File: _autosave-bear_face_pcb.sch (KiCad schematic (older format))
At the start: 201 parts, among them J1 GT-USB-7010EN, J2 Conn_02x03_Odd_Even, SW1 RESET, U1 ATmega32U4-AU, U2 SRV05-4, Y1 16MHz

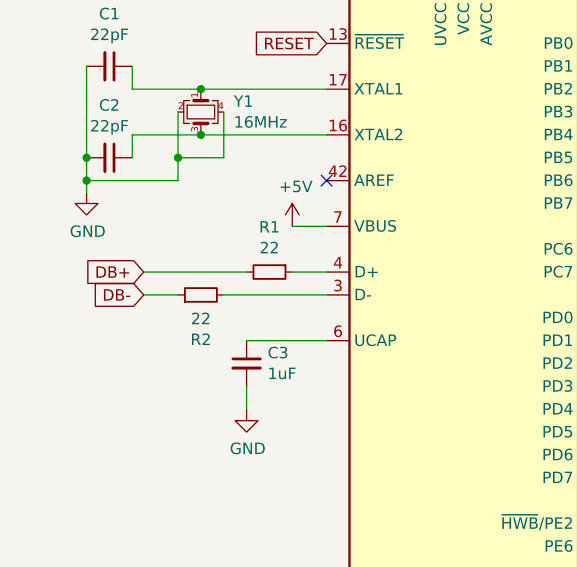
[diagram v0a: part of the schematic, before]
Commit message: initial USB-C commit
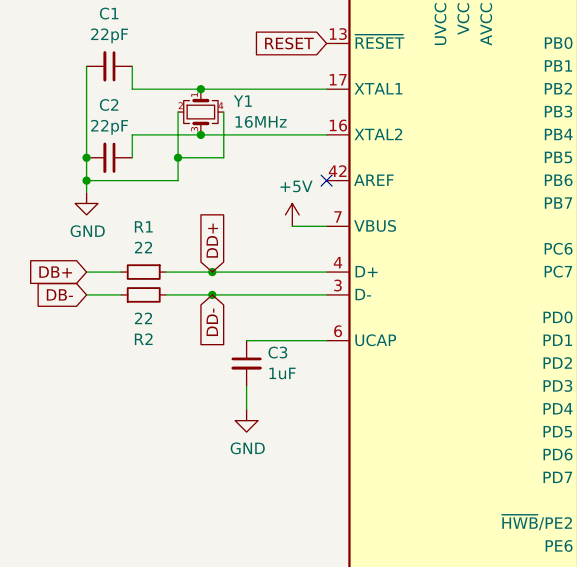
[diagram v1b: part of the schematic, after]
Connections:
- net DD-: now reaches R2.2, U1.3 (D-)
- net DD+: now reaches R1.1, U1.4 (D+)
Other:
- moved on the sheet: R1, R2
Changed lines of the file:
@@
 Text GLabel 5500 5900 2    50   Input ~ 0
 DA+
-Text GLabel 1550 2450 0    50   Input ~ 0
-DB-
 Text GLabel 3300 3500 1    50   Input ~ 0
 LEDPIN
-Text GLabel 950  5150 0    50   Input ~ 0
-DB+
-Text GLabel 950  5250 0    50   Input ~ 0
-DB-
 Wire Wire Line
 	2250 7450 2350 7450
@@
 Wire Wire Line
 	1700 2600 1550 2600
-Text GLabel 1550 2600 0    50   Input ~ 0
-DB+
 Wire Wire Line
 	1700 2250 1700 2600
@@
 L Device:R_Small R1
 U 1 1 66036275
-P 1500 5150
-F 0 "R1" V 1304 5150 50  0000 C CNN
-F 1 "22" V 1395 5150 50  0000 C CNN
-F 2 "Resistor_SMD:R_0805_2012Metric" H 1500 5150 50  0001 C CNN
-F 3 "~" H 1500 5150 50  0001 C CNN
-	1    1500 5150
+P 950 5150
+F 0 "R1" V 754 5150 50  0000 C CNN
+F 1 "22" V 845 5150 50  0000 C CNN
+F 2 "Resistor_SMD:R_0805_2012Metric" H 950 5150 50  0001 C CNN
+F 3 "~" H 950 5150 50  0001 C CNN
+	1    950  5150
 	0    1    1    0
 $EndComp
-Wire Wire Line
-	1750 5150 1600 5150
-Wire Wire Line
-	1400 5150 950  5150
-Wire Wire Line
-	1100 5250 950  5250
-Wire Wire Line
-	1300 5250 1750 5250
 $Comp
 L Device:R_Small R2
 U 1 1 66037A5E
-P 1200 5250
-F 0 "R2" V 1004 5250 50  0000 C CNN
-F 1 "22" V 1095 5250 50  0000 C CNN
-F 2 "Resistor_SMD:R_0805_2012Metric" H 1200 5250 50  0001 C CNN
-F 3 "~" H 1200 5250 50  0001 C CNN
-	1    1200 5250
+P 950 5250
+F 0 "R2" V 754 5250 50  0000 C CNN
+F 1 "22" V 845 5250 50  0000 C CNN
+F 2 "Resistor_SMD:R_0805_2012Metric" H 950 5250 50  0001 C CNN
+F 3 "~" H 950 5250 50  0001 C CNN
+	1    950  5250
 	0    -1   -1   0
 $EndComp
+Text GLabel 700  5250 0    50   Input ~ 0
+DB-
+Text GLabel 700  5150 0    50   Input ~ 0
+DB+
+Text GLabel 1550 2600 0    50   Input ~ 0
+DB+
+Text GLabel 1550 2450 0    50   Input ~ 0
+DB-
+Text GLabel 1250 5150 1    50   Input ~ 0
+DD+
+Wire Wire Line
+	700  5150 850  5150
+Wire Wire Line
+	1050 5150 1250 5150
+Wire Wire Line
+	700  5250 850  5250
+Wire Wire Line
+	1050 5250 1250 5250
+Connection ~ 1250 5150
+Wire Wire Line
+	1250 5150 1750 5150
+Connection ~ 1250 5250
+Wire Wire Line
+	1250 5250 1750 5250
+Text GLabel 1250 5250 3    50   Input ~ 0
+DD-
 $EndSCHEMATC
